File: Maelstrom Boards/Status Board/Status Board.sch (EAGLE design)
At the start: 32 parts, among them IC1 LM555D, P1 39-30-04, Q1 310mA/60V/1.6Ω, Q2 310mA/60V/1.6Ω

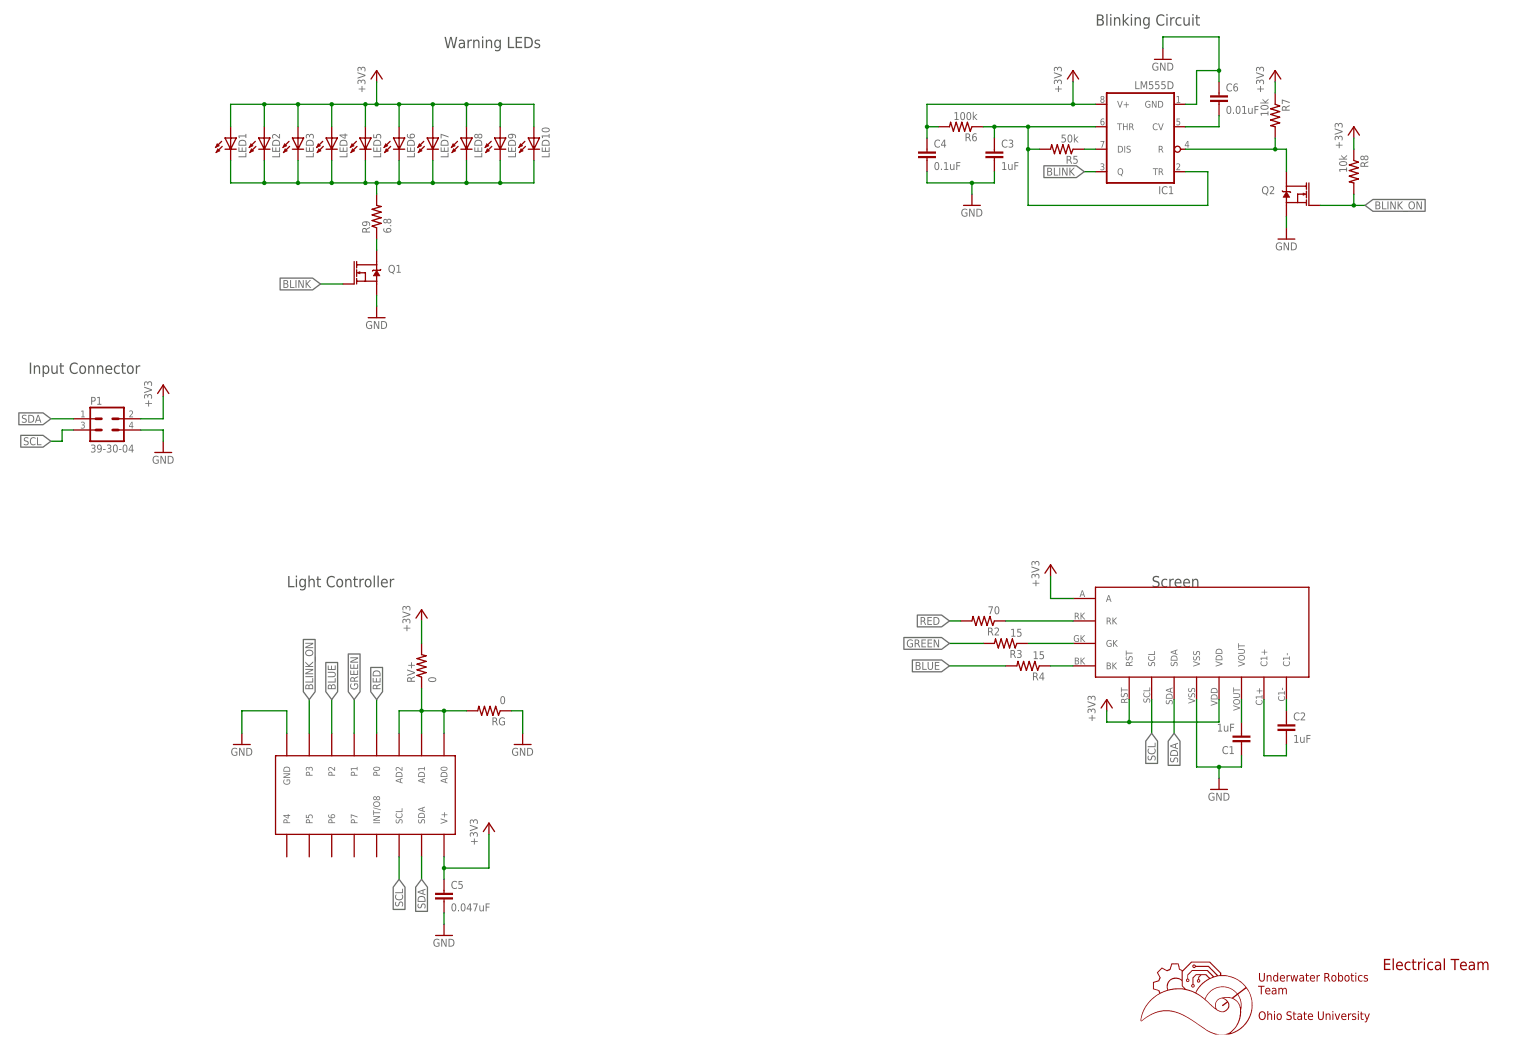
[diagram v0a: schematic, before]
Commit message: Final changes before order
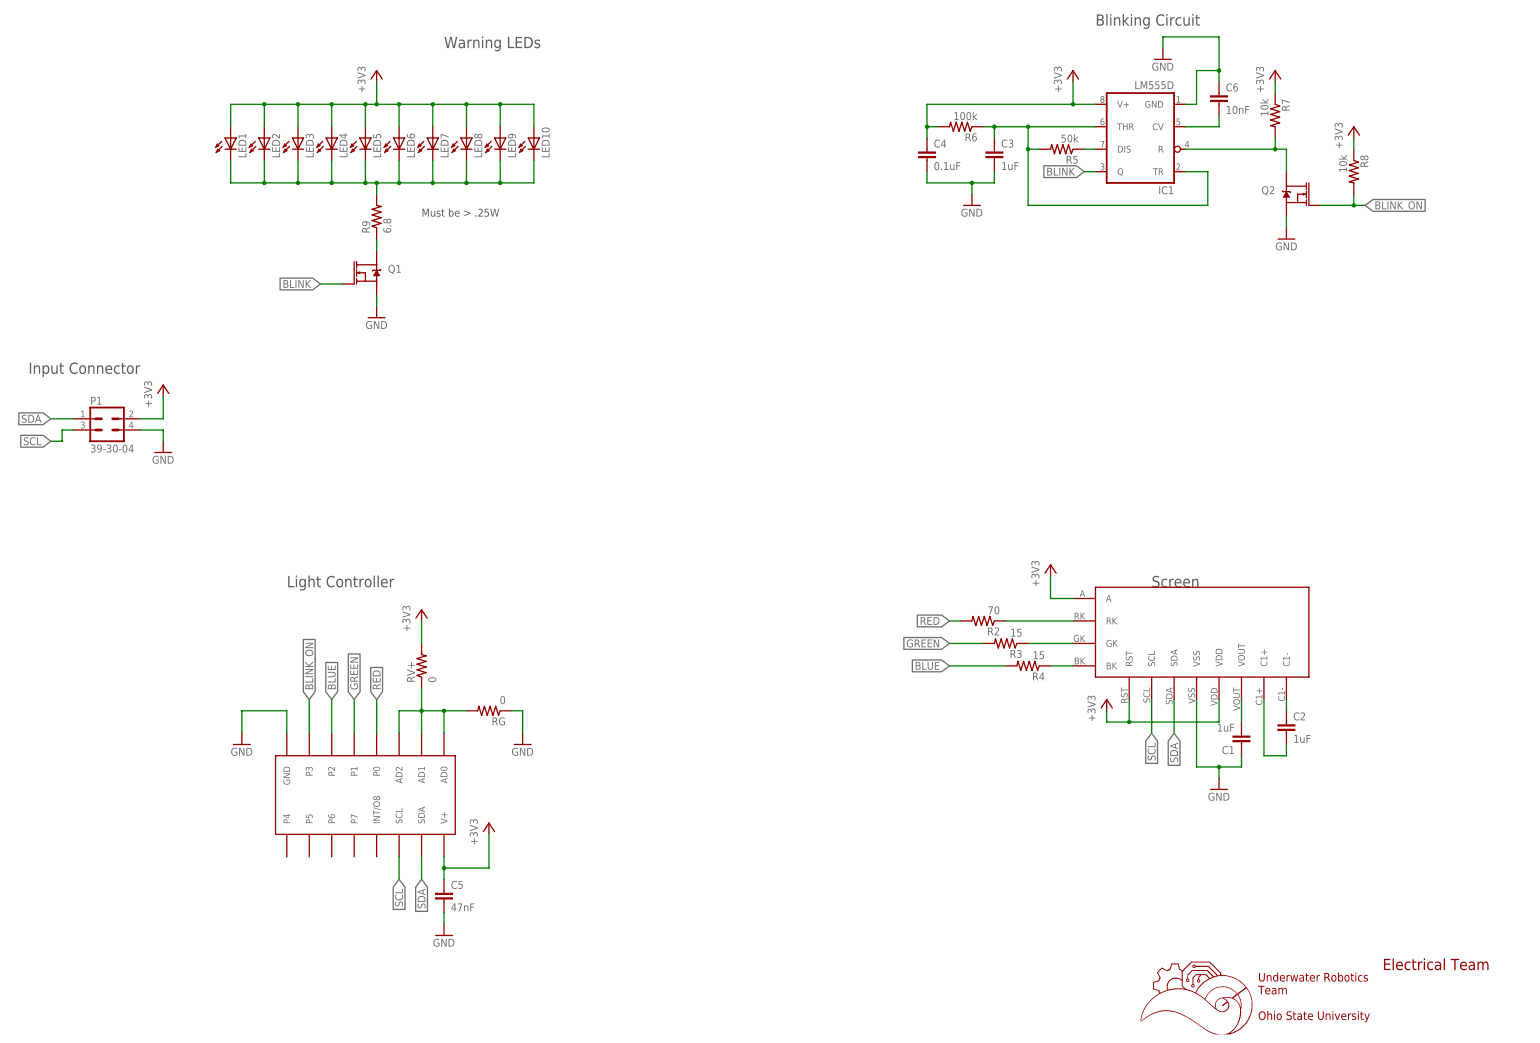
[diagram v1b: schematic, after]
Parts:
- C5: value 0.047uF -> 47nF
- C6: value 0.01uF -> 10nF
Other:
- note added: "Must be > .25W"
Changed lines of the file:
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@@
 <part name="Q1" library="SparkFun-DiscreteSemi" library_urn="urn:adsk.eagle:library:514" deviceset="MOSFET-NCH" device="-2N7002PW" package3d_urn="urn:adsk.eagle:package:38456/1" value="310mA/60V/1.6Ω"/>
 <part name="GND3" library="supply1" library_urn="urn:adsk.eagle:library:371" deviceset="GND" device=""/>
-<part name="C5" library="rcl" library_urn="urn:adsk.eagle:library:334" deviceset="C-EU" device="C0603" package3d_urn="urn:adsk.eagle:package:23616/2" value="0.047uF"/>
+<part name="C5" library="rcl" library_urn="urn:adsk.eagle:library:334" deviceset="C-EU" device="C0603" package3d_urn="urn:adsk.eagle:package:23616/2" value="47nF"/>
 <part name="GND8" library="supply1" library_urn="urn:adsk.eagle:library:371" deviceset="GND" device=""/>
-<part name="C6" library="rcl" library_urn="urn:adsk.eagle:library:334" deviceset="C-EU" device="C0603" package3d_urn="urn:adsk.eagle:package:23616/2" value="0.01uF"/>
+<part name="C6" library="rcl" library_urn="urn:adsk.eagle:library:334" deviceset="C-EU" device="C0603" package3d_urn="urn:adsk.eagle:package:23616/2" value="10nF"/>
 <part name="Q2" library="SparkFun-DiscreteSemi" library_urn="urn:adsk.eagle:library:514" deviceset="MOSFET-NCH" device="-2N7002PW" package3d_urn="urn:adsk.eagle:package:38456/1" value="310mA/60V/1.6Ω"/>
 <part name="R8" library="rcl" library_urn="urn:adsk.eagle:library:334" deviceset="R-US_" device="R0603" package3d_urn="urn:adsk.eagle:package:23555/2" value="10k"/>
@@
 <text x="96.52" y="106.68" size="2.54" layer="97">Light Controller</text>
 <text x="38.1" y="154.94" size="2.54" layer="97">Input Connector</text>
+<text x="127" y="190.5" size="1.778" layer="97">Must be &gt; .25W</text>
 </plain>
 <instances>
